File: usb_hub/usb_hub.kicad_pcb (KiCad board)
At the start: 2 copper layers, 100 x 21 mm, 147 parts, among them Q1 2N3904, U1 TPS2044B, U10 USB_A_FEMALE, U11 USB_A_FEMALE, U12 SN75240, U13 SN75240, U14 M93C46, U15 USB_A_FEMALE, U16 USB_A_FEMALE, U17 USB_A_FEMALE, U18 USB_A_FEMALE, U2 TPS2044B, U3 TUSB2077A, U4 TPS76333, U5 USB_A_MALE, U6 SN75240, U7 SN75240, U8 SN75240, U9 USB_A_FEMALE, X1 6 MHz

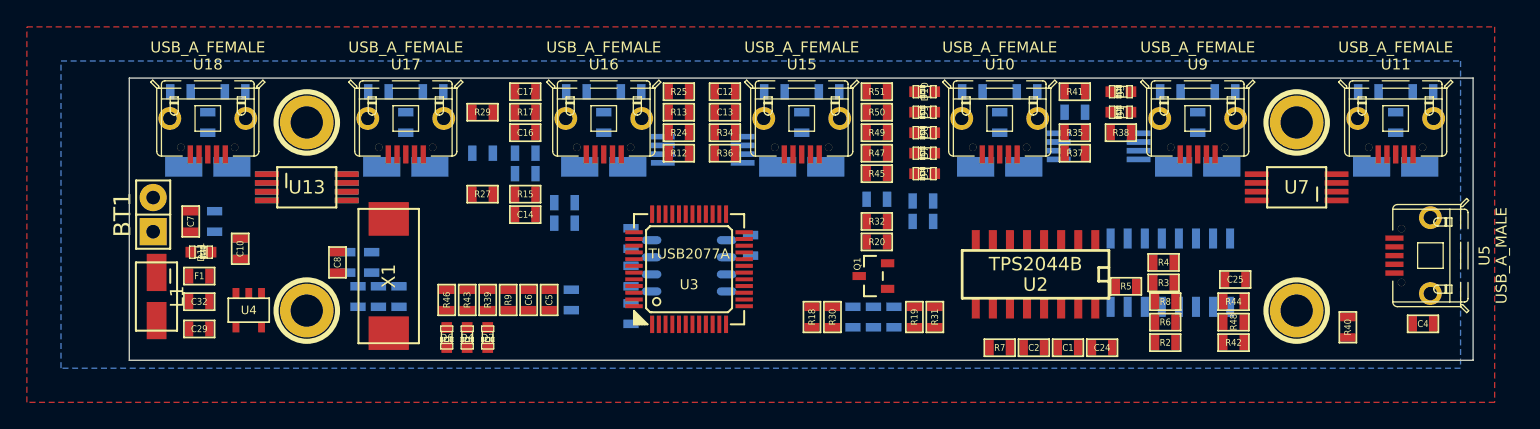
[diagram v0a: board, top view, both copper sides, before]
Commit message: finished the usb_hub
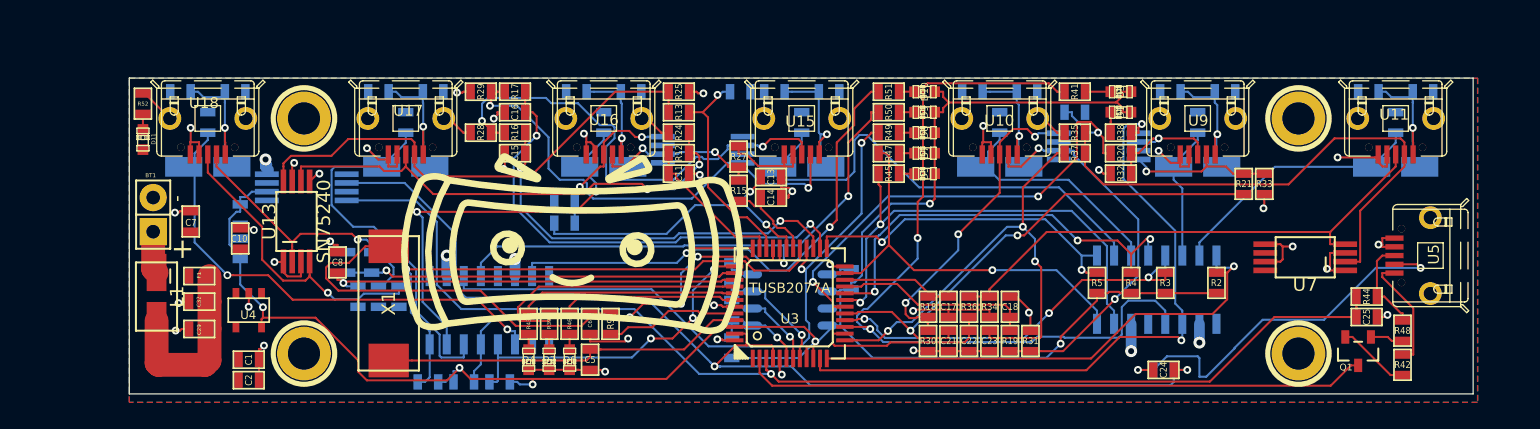
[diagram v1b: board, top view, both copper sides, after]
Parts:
- added G***: LOGO, logo:logo, F.Cu at (68.5, 41.5)
- C11, C15, C18, C21, C22, C23, R16, R21, R28, R33, R52: moved to F.Cu
- C12, C4, R40, R6, R7, R8, U2: moved to B.Cu
- moved C4 88.4 mm to (43.8, 39.4), turned to 270 degrees
- moved C1 61.0 mm to (44.5, 50.2)
- moved C2 58.5 mm to (44.5, 51.7), turned to 0 degrees
- moved R6 55.0 mm to (57.8, 51.8), turned to 180 degrees
- moved R8 49.9 mm to (63.1, 51.8), turned to 180 degrees
- moved U2 40.7 mm to (62.4, 46.5), turned to 0 degrees
- moved R7 40.0 mm to (60.5, 51.8), turned to 0 degrees
- moved Q1 36.5 mm to (127.0, 49.5), turned to 180 degrees
- moved C17 35.3 mm to (96.5, 46.2), turned to 270 degrees
- moved R33 25.6 mm to (120.0, 37.1), turned to 90 degrees
- moved R21 23.9 mm to (118.5, 37.1), turned to 90 degrees
- moved R34 23.6 mm to (99.6, 46.2), turned to 90 degrees
- moved R36 21.5 mm to (98.0, 46.2), turned to 90 degrees
- moved R20 19.3 mm to (109.3, 34.8)
- moved R27 19.3 mm to (80.9, 35.1), turned to 270 degrees
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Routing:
- net 3.3V: track 0.00 -> 149.7 mm, vias 0 -> 6
- net GND: track 0.00 -> 111.7 mm, vias 0 -> 38
- net DP0: track 0.00 -> 88.3 mm, vias 0 -> 1
- net DM0: track 0.00 -> 80.8 mm, vias 0 -> 2
- net PWRON2: track 0.00 -> 59.9 mm, vias 0 -> 2
- net PWRON1: track 0.00 -> 49.3 mm, vias 0 -> 2
- net PWRON5: track 0.00 -> 48.7 mm, vias 0 -> 2
- net DP0PUR: track 0.00 -> 46.6 mm
- net PWRON7: track 0.00 -> 42.5 mm, vias 0 -> 2
- net OC5: track 0.00 -> 40.8 mm, vias 0 -> 1
- net PWRON6: track 0.00 -> 40.5 mm, vias 0 -> 2
- net DM1: track 0.00 -> 39.7 mm
- net DP1: track 0.00 -> 39.0 mm
- net Net-(C21-Pad1): track 0.00 -> 38.1 mm, vias 0 -> 2
- net Net-(C19-Pad1): track 0.00 -> 37.4 mm, vias 0 -> 3
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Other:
- board size 100 x 21 mm -> 100 x 23.5 mm
- net class Default: clearance 0.254 -> 0.1524; trace_width 0.254 -> 0.1524
- net class VCC added: clearance 0.1524, trace_width 0.8, via_dia 0.889, via_drill 0.635
- rule trace_clearance: 0.254 -> 0.1524
- board text added: "+"
- board text added: "-"
